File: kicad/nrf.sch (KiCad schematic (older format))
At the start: 6 parts, among them P1 ICSP, P2 CONN_01X02, P3 NRF_24L01, U1 MCP1755ST-3302E/DB

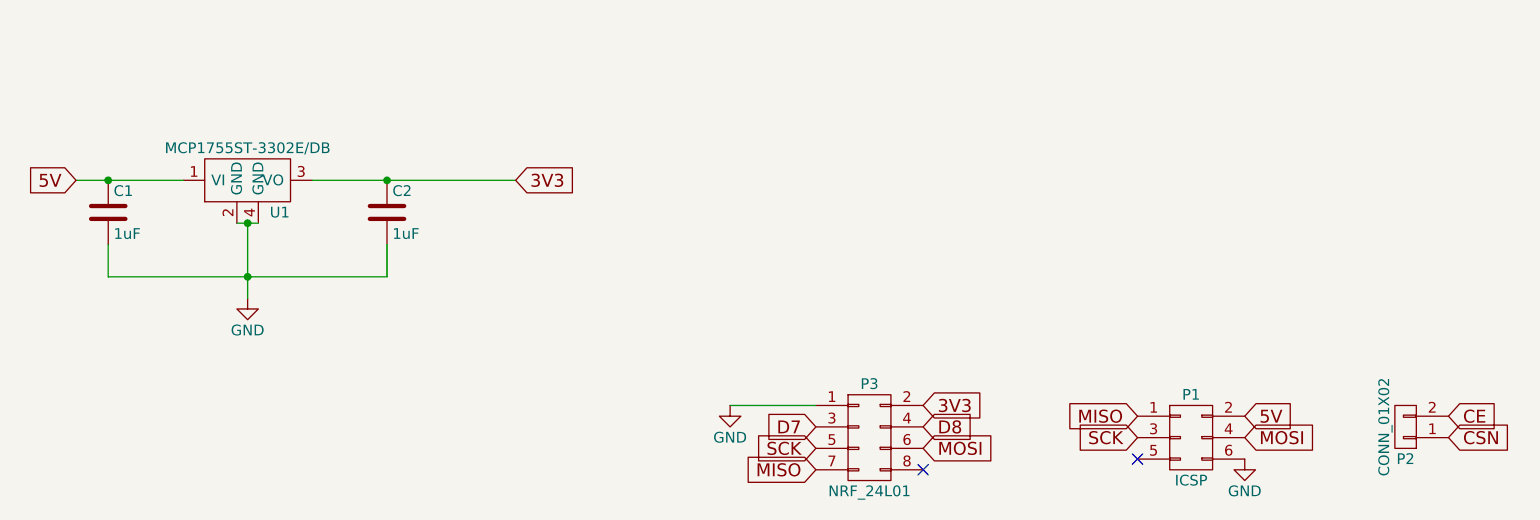
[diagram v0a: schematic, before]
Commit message: Voltage regulator
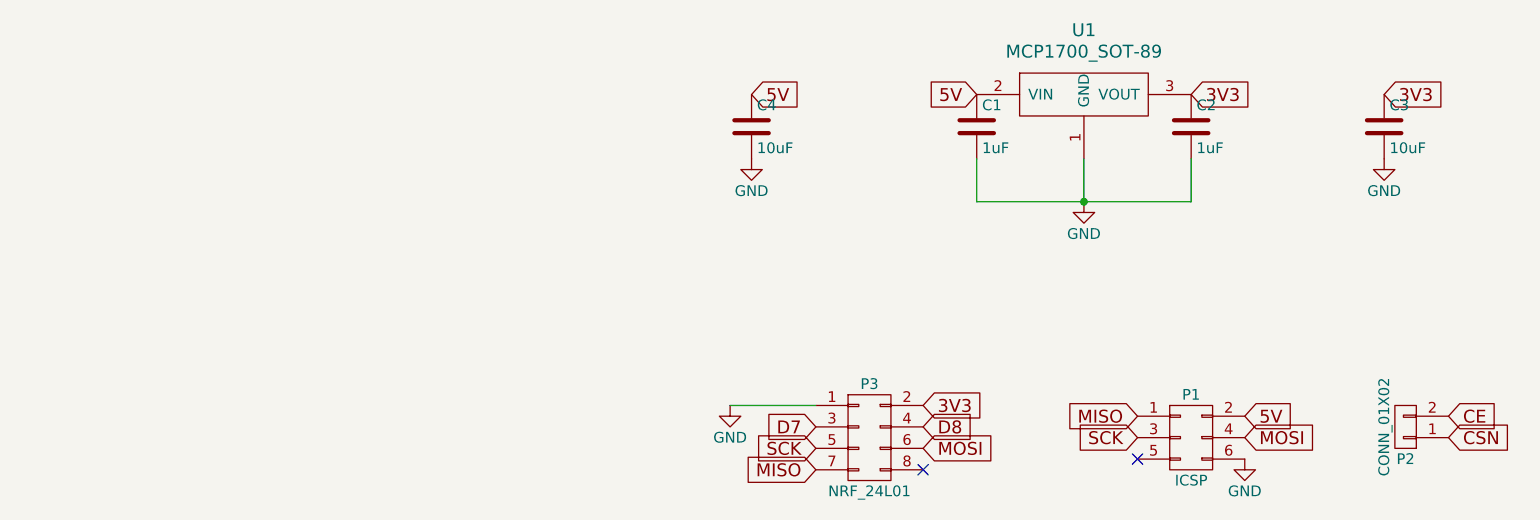
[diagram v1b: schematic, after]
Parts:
- removed U1: MCP1755ST-3302E/DB, TO_SOT_Packages_SMD:SOT-223, symbol MCP1755ST-3302E/DB
- added C3, C4: 10uF, Capacitors_SMD:C_0805_HandSoldering, symbol C
- added U1: MCP1700_SOT-89, TO_SOT_Packages_SMD:SOT89-3_Housing_Handsoldering, symbol MCP1700_SOT-89
- P3: footprint Socket_Strips:Socket_Strip_Straight_2x04 -> nrf:NRF_24L01
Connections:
- net 3V3: now also C3.1, U1.3 (VOUT)
- net 5V: now also C4.1, U1.2 (VIN)
- net GND: now also C3.2, C4.2, U1.1 (GND)
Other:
- moved on the sheet: C1, C2
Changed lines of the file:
@@
 LIBS:contrib
 LIBS:valves
+LIBS:nrf
 LIBS:nrf-cache
-LIBS:rc_power_sockets-cache
 EELAYER 25 0
 EELAYER END
@@
 F 0 "P3" H 5700 4000 50  0000 C CNN
 F 1 "NRF_24L01" H 5700 3500 50  0000 C CNN
-F 2 "Socket_Strips:Socket_Strip_Straight_2x04" H 5700 2550 50  0001 C CNN
+F 2 "nrf:NRF_24L01" H 5700 2550 50  0001 C CNN
 F 3 "" H 5700 2550 50  0000 C CNN
 	1    5700 3750
@@
 L GND #PWR03
 U 1 1 571F9F29
-P 2800 3100
-F 0 "#PWR03" H 2800 2850 50  0001 C CNN
-F 1 "GND" H 2800 2950 50  0000 C CNN
-F 2 "" H 2800 3100 50  0000 C CNN
-F 3 "" H 2800 3100 50  0000 C CNN
-	1    2800 3100
+P 6700 2650
+F 0 "#PWR03" H 6700 2400 50  0001 C CNN
+F 1 "GND" H 6700 2500 50  0000 C CNN
+F 2 "" H 6700 2650 50  0000 C CNN
+F 3 "" H 6700 2650 50  0000 C CNN
+	1    6700 2650
 	1    0    0    -1
 $EndComp
@@
 L C C2
 U 1 1 571F9F2B
-P 3450 2700
-F 0 "C2" H 3475 2800 50  0000 L CNN
-F 1 "1uF" H 3475 2600 50  0000 L CNN
-F 2 "Capacitors_SMD:C_0805_HandSoldering" H 3488 2550 50  0001 C CNN
-F 3 "" H 3450 2700 50  0000 C CNN
-	1    3450 2700
+P 7200 2300
+F 0 "C2" H 7225 2400 50  0000 L CNN
+F 1 "1uF" H 7225 2200 50  0000 L CNN
+F 2 "Capacitors_SMD:C_0805_HandSoldering" H 7238 2150 50  0001 C CNN
+F 3 "" H 7200 2300 50  0000 C CNN
+	1    7200 2300
 	1    0    0    -1
 $EndComp
@@
 L C C1
 U 1 1 571F9F2C
-P 2150 2700
-F 0 "C1" H 2175 2800 50  0000 L CNN
-F 1 "1uF" H 2175 2600 50  0000 L CNN
-F 2 "Capacitors_SMD:C_0805_HandSoldering" H 2188 2550 50  0001 C CNN
-F 3 "" H 2150 2700 50  0000 C CNN
-	1    2150 2700
-	1    0    0    -1
-$EndComp
-Wire Wire Line
-	2000 2550 2500 2550
-Connection ~ 2150 2550
-Wire Wire Line
-	3100 2550 4050 2550
-Wire Wire Line
-	2800 2750 2800 3100
-Wire Wire Line
-	2150 2850 2150 3000
-Wire Wire Line
-	2150 3000 3450 3000
-Connection ~ 2800 3000
-Wire Wire Line
-	3450 3000 3450 2850
-Connection ~ 3450 2550
-$Comp
-L MCP1755ST-3302E/DB U1
-U 1 1 571F9F50
-P 2800 2550
-F 0 "U1" H 2950 2400 50  0000 C CNN
-F 1 "MCP1755ST-3302E/DB" H 2800 2700 50  0000 C CNN
-F 2 "TO_SOT_Packages_SMD:SOT-223" H 2800 2550 50  0001 C CNN
-F 3 "" H 2800 2550 50  0000 C CNN
-	1    2800 2550
-	1    0    0    -1
-$EndComp
-Wire Wire Line
-	2750 2750 2850 2750
-Connection ~ 2800 2750
-Text GLabel 2000 2550 0    60   Input ~ 0
+P 6200 2300
+F 0 "C1" H 6225 2400 50  0000 L CNN
+F 1 "1uF" H 6225 2200 50  0000 L CNN
+F 2 "Capacitors_SMD:C_0805_HandSoldering" H 6238 2150 50  0001 C CNN
+F 3 "" H 6200 2300 50  0000 C CNN
+	1    6200 2300
+	1    0    0    -1
+$EndComp
+Text GLabel 6200 2150 0    60   Input ~ 0
 5V
-Text GLabel 4050 2550 2    60   Input ~ 0
+Text GLabel 7200 2150 2    60   Input ~ 0
 3V3
+$Comp
+L MCP1700_SOT-89 U1
+U 1 1 5720ABAB
+P 6700 1950
+F 0 "U1" H 6700 2050 60  0000 C CNN
+F 1 "MCP1700_SOT-89" H 6700 1950 60  0000 C CNN
+F 2 "TO_SOT_Packages_SMD:SOT89-3_Housing_Handsoldering" H 6700 1950 60  0001 C CNN
+F 3 "" H 6700 1950 60  0000 C CNN
+	1    6700 1950
+	1    0    0    -1
+$EndComp
+Wire Wire Line
+	6700 2450 6700 2650
+Wire Wire Line
+	7200 2650 7200 2450
+Wire Wire Line
+	6200 2650 7200 2650
+Wire Wire Line
+	6200 2450 6200 2650
+Connection ~ 6700 2650
+$Comp
+L C C3
+U 1 1 5720B5A0
+P 8100 2300
+F 0 "C3" H 8125 2400 50  0000 L CNN
+F 1 "10uF" H 8125 2200 50  0000 L CNN
+F 2 "Capacitors_SMD:C_0805_HandSoldering" H 8138 2150 50  0001 C CNN
+F 3 "" H 8100 2300 50  0000 C CNN
+	1    8100 2300
+	1    0    0    -1
+$EndComp
+Text GLabel 8100 2150 2    60   Input ~ 0
+3V3
+$Comp
+L GND #PWR04
+U 1 1 5720B66D
+P 8100 2450
+F 0 "#PWR04" H 8100 2200 50  0001 C CNN
+F 1 "GND" H 8100 2300 50  0000 C CNN
+F 2 "" H 8100 2450 50  0000 C CNN
+F 3 "" H 8100 2450 50  0000 C CNN
+	1    8100 2450
+	1    0    0    -1
+$EndComp
+$Comp
+L C C4
+U 1 1 5720B905
+P 5150 2300
+F 0 "C4" H 5175 2400 50  0000 L CNN
+F 1 "10uF" H 5175 2200 50  0000 L CNN
+F 2 "Capacitors_SMD:C_0805_HandSoldering" H 5188 2150 50  0001 C CNN
+F 3 "" H 5150 2300 50  0000 C CNN
+	1    5150 2300
+	1    0    0    -1
+$EndComp
+Text GLabel 5150 2150 2    60   Input ~ 0
+5V
+$Comp
+L GND #PWR05
+U 1 1 5720B90C
+P 5150 2450
+F 0 "#PWR05" H 5150 2200 50  0001 C CNN
+F 1 "GND" H 5150 2300 50  0000 C CNN
+F 2 "" H 5150 2450 50  0000 C CNN
+F 3 "" H 5150 2450 50  0000 C CNN
+	1    5150 2450
+	1    0    0    -1
+$EndComp
 $EndSCHEMATC

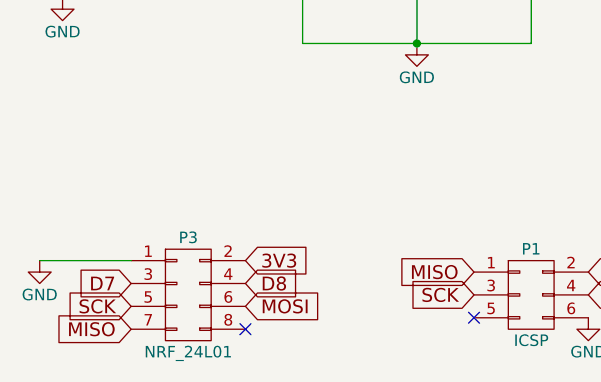
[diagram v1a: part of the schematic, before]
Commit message: Traces
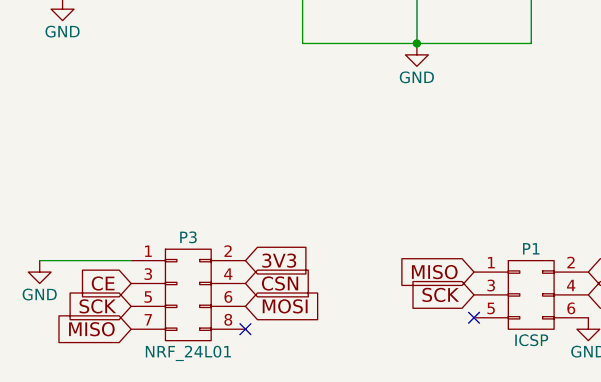
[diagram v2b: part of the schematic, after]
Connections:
- net D7 is gone; now on net CE: P3.3 (P3)
- net D8 is gone; now on net CSN: P3.4 (P4)
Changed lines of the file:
@@
 	1    0    0    -1
 $EndComp
-Text GLabel 5450 3700 0    60   Input ~ 0
-D7
 Text GLabel 5450 3800 0    60   Input ~ 0
 SCK
@@
 Text GLabel 5950 3800 2    60   Input ~ 0
 MOSI
-Text GLabel 5950 3700 2    60   Input ~ 0
-D8
 Text GLabel 5950 3600 2    60   Input ~ 0
 3V3
@@
 	1    0    0    -1
 $EndComp
+Text GLabel 5450 3700 0    60   Input ~ 0
+CE
+Text GLabel 5950 3700 2    60   Input ~ 0
+CSN
 $EndSCHEMATC
